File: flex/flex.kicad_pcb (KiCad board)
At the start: 2 copper layers, 47.2 x 41.5 mm, 9 parts, among them J1 Conn_01x06_Female, SW19 SW_Push, SW5 SW_Push, SW9 SW_Push

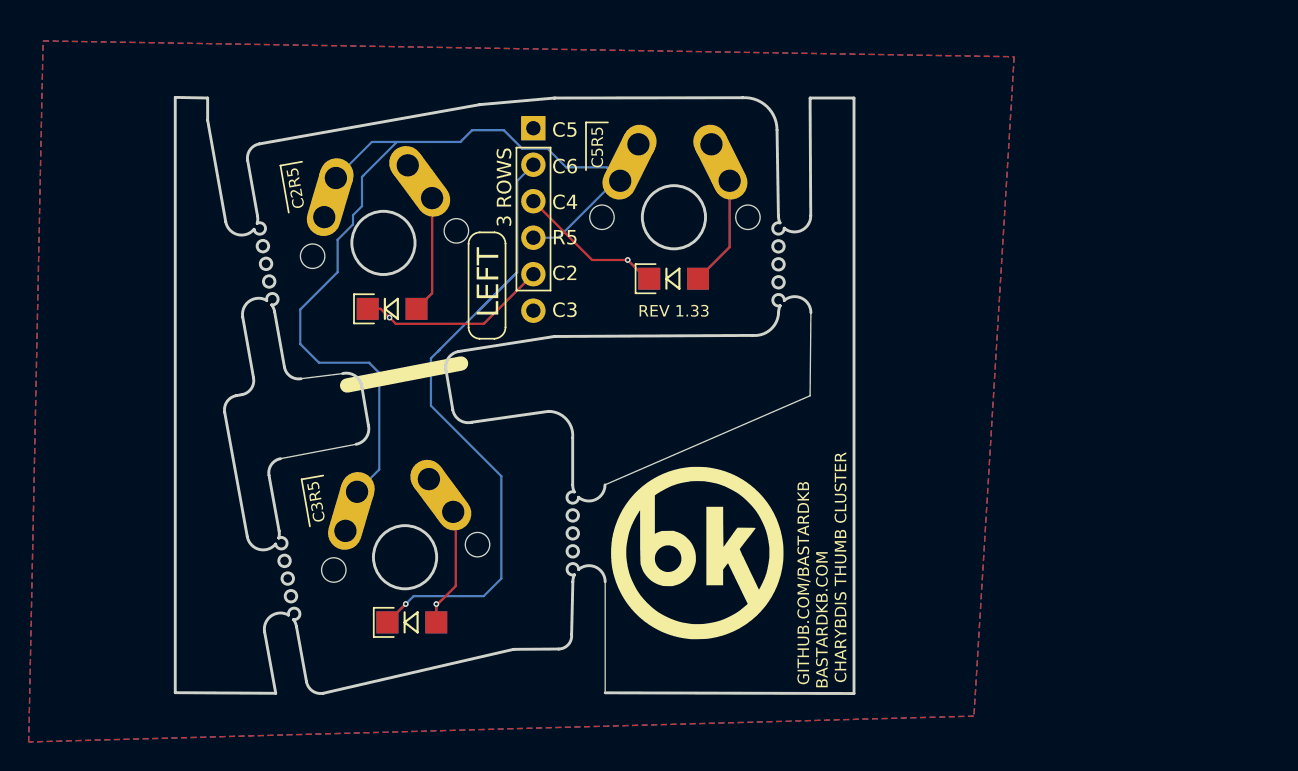
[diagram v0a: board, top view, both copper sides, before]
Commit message: add rgb
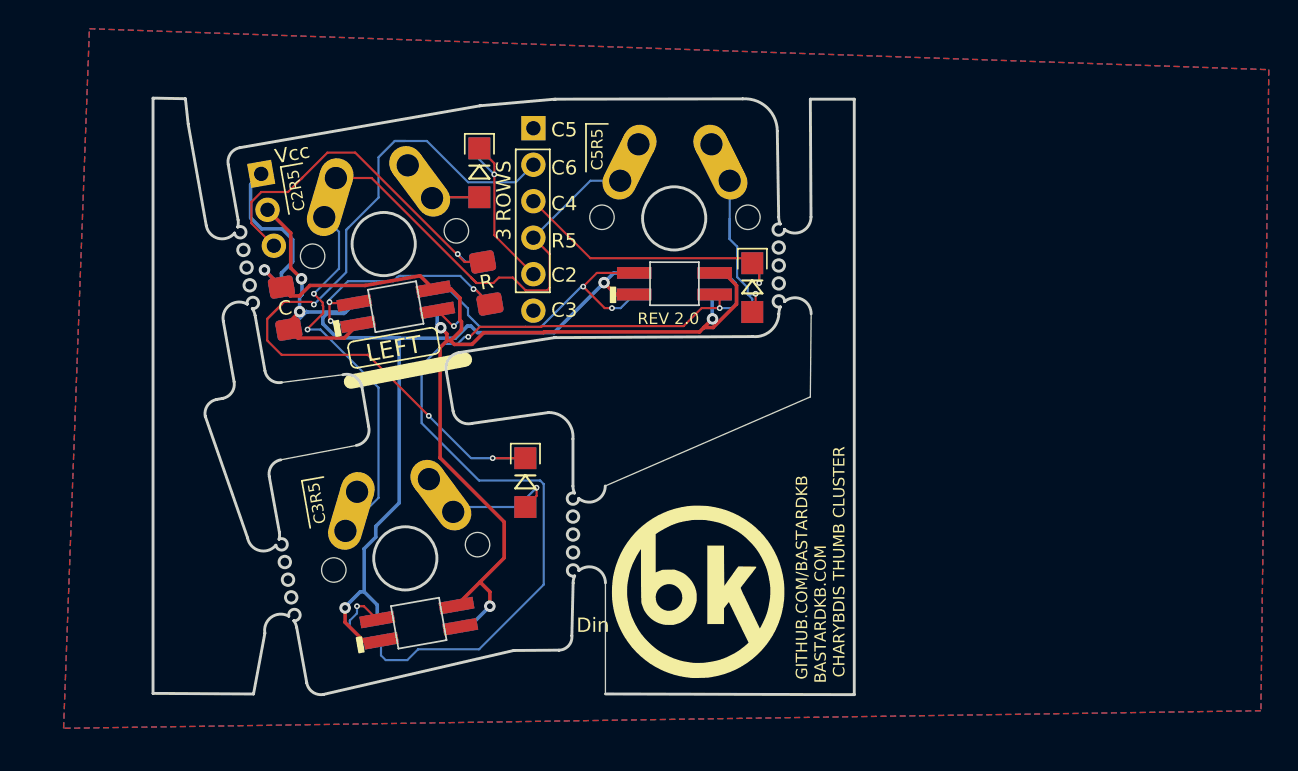
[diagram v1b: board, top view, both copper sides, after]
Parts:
- removed the G*** at (95.8, 98.0)
- removed the G*** at (95.9, 98.0)
- added C1: C, LED_SMD:LED_1206_3216Metric_Pad1.42x1.75mm_HandSolder, F.Cu at (67.2, 80.9)
- added C2: C, LED_SMD:LED_1206_3216Metric_Pad1.42x1.75mm_HandSolder, B.Cu at (67.2, 80.9)
- added D10: SK6812MINI, libs2:YS-SK6812MINI-E_REVERSE, F.Cu at (94.2, 79.2)
- added D11: SK6812MINI, libs2:YS-SK6812MINI-E_REVERSE_NO_EDGECUT, B.Cu at (94.2, 79.2)
- added D12: SK6812MINI, libs2:YS-SK6812MINI-E_REVERSE, F.Cu at (74.8, 80.8)
- added D13: SK6812MINI, libs2:YS-SK6812MINI-E_REVERSE_NO_EDGECUT, B.Cu at (74.8, 80.8)
- added D2: SK6812MINI, libs2:YS-SK6812MINI-E_REVERSE, F.Cu at (76.5, 102.8)
- added D3: SK6812MINI, libs2:YS-SK6812MINI-E_REVERSE_NO_EDGECUT, B.Cu at (76.5, 102.8)
- added G***: LOGO, LOGO, F.Cu at (95.9, 100.7)
- added G***: LOGO, LOGO, B.Cu at (96.0, 100.7)
- added J2: Conn_01x03_Female, Connector_PinHeader_2.54mm:PinHeader_1x03_P2.54mm_Vertical, F.Cu at (65.5, 71.6)
- added R1: R, Resistor_SMD:R_1206_3216Metric_Pad1.42x1.75mm_HandSolder, B.Cu at (81.1, 79.1)
- added R2: R, Resistor_SMD:R_1206_3216Metric_Pad1.42x1.75mm_HandSolder, F.Cu at (81.2, 79.2)
- moved D9 19.6 mm to (83.9, 88.0), turned to -90 degrees
- moved D5 18.2 mm to (80.7, 66.5), turned to -90 degrees
- moved D19 11.4 mm to (99.7, 74.5), turned to -90 degrees
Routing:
- net Vcc: track 0.00 -> 87.1 mm, vias 0 -> 4
- net Gnd: track 0.00 -> 77.7 mm, vias 0 -> 4
- net Net-(D10-Pad1): track 0.00 -> 69.9 mm, vias 0 -> 3
- net Net-(D12-Pad1): track 0.00 -> 28.0 mm, vias 0 -> 3
- net Din: track 0.00 -> 26.4 mm, vias 0 -> 1
- net Net-(D12-Pad3): track 0.00 -> 19.5 mm, vias 0 -> 3
- net Net-(D5-Pad2): track 16.3 -> 6.63 mm
- net col4: track 12.3 -> 20.2 mm
- net col6: track 48.7 -> 56.4 mm, vias 1 -> 3
- net row1: track 62.8 -> 57.9 mm, vias 0 -> 2
- net col2: track 15.2 -> 12.7 mm
- net Net-(D19-Pad2): track 15.5 -> 13.1 mm, vias 0 -> 1
- net Net-(D9-Pad2): track 10.1 -> 8.50 mm
- added copper zone on B.Cu, net Gnd
- added copper zone on F.Cu, net Gnd
- removed copper zone on B.Cu, net (none)
- removed copper zone on F.Cu, net (none)
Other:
- board size 47.2 x 41.5 mm -> 48.8 x 41.5 mm
- board text added: "C"
- board text added: "Conn_01x02_Female"
- board text added: "Conn_01x06_Female"
- board text added: "Din"
- board text added: "R"
- board text added: "REV 2.0"
- board text added: "Vcc"
- board text removed: "REV 1.33"
